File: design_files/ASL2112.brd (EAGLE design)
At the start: 11.5 x 15.3 mm, 14 parts, among them J1 47346-0001, J2 SM02B-SRSS-TB(LF)(SN), J3 PIN_1X.1"1, J4 PIN_1X.1"1, U1 MCP73831

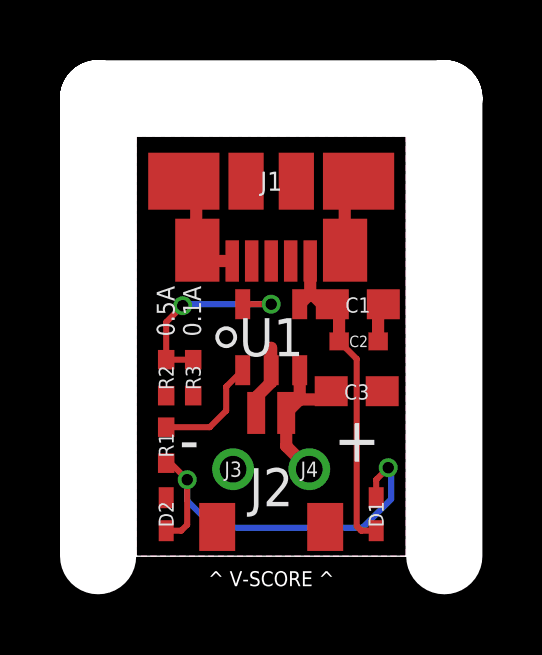
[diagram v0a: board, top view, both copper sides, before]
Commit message: update format
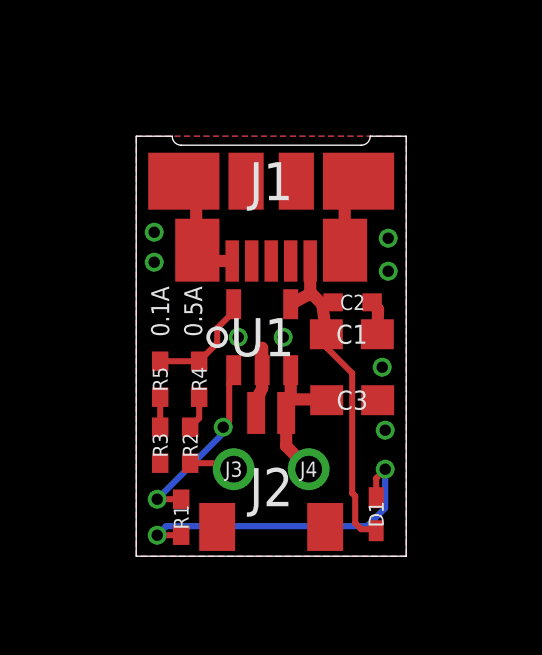
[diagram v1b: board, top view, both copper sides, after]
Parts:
- removed D2: GREEN, tinycircuits:0402_LED
- added R4, R5: 0.0, tinycircuits:0402
- D1: value RED -> AMBER
- moved R3 2.50 mm to (16.3, 14.7), turned to 270 degrees
- moved R1 2.45 mm to (17.0, 12.3)
- moved R2 2.39 mm to (17.3, 14.7), turned to 270 degrees
- moved C2 1.32 mm to (22.7, 19.5)
- moved C1 1.02 mm to (22.7, 18.4)
- moved C3 0.34 mm to (22.7, 16.2)
- moved U1 0.30 mm to (19.7, 18.3)
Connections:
- new net N$4: R2.1, R4.2
- new net N$7: R3.1, R5.2
- net GND: now also R2.2, R3.2; no longer D2.2, R2.1, R3.1
- net N$2: no longer D2.1
- net N$3: now also R4.1, R5.1; no longer R2.2, R3.2
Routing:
- net N$3: track 6.85 -> 3.68 mm, vias 2 -> 0
- net N$2: track 13.7 -> 11.1 mm
- net N$1: track 3.81 -> 6.12 mm, vias 0 -> 2
- net GND: track 8.62 -> 9.80 mm, vias 0 -> 8
- net N$4: track 0.00 -> 1.12 mm
- net N$7: track 0.00 -> 1.00 mm
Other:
- board size 11.5 x 15.3 mm -> 9 x 14 mm
- board text added: "2"
- board text added: "ASL2112 - Rev2"
- board text removed: "1"
- board text removed: "ASL2112 - Rev1"
- board text removed: "^ V-SCORE ^"
